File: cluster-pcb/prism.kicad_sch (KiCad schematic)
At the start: 8 parts, among them J501 Conn_01x04_P3.5mm_TBH_Horizon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, U501 Interface_RS485_MAX13431E, U502 TPS1H200AQDGNRQ1

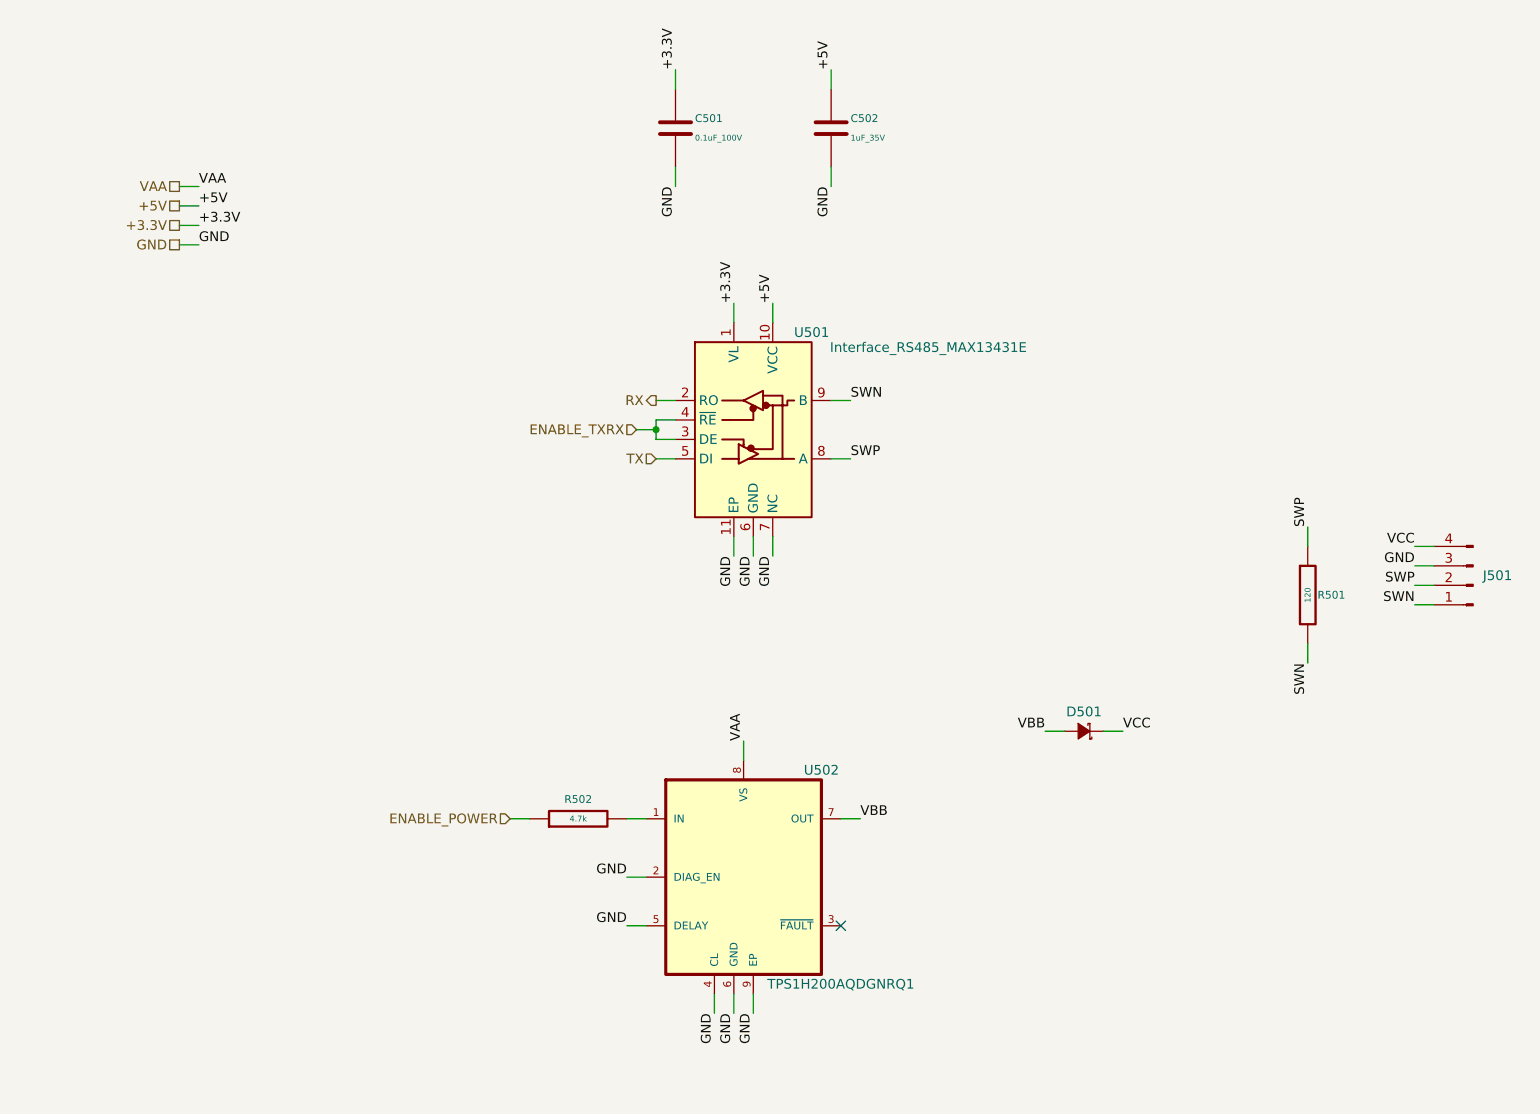
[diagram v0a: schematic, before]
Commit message: First SPI changes
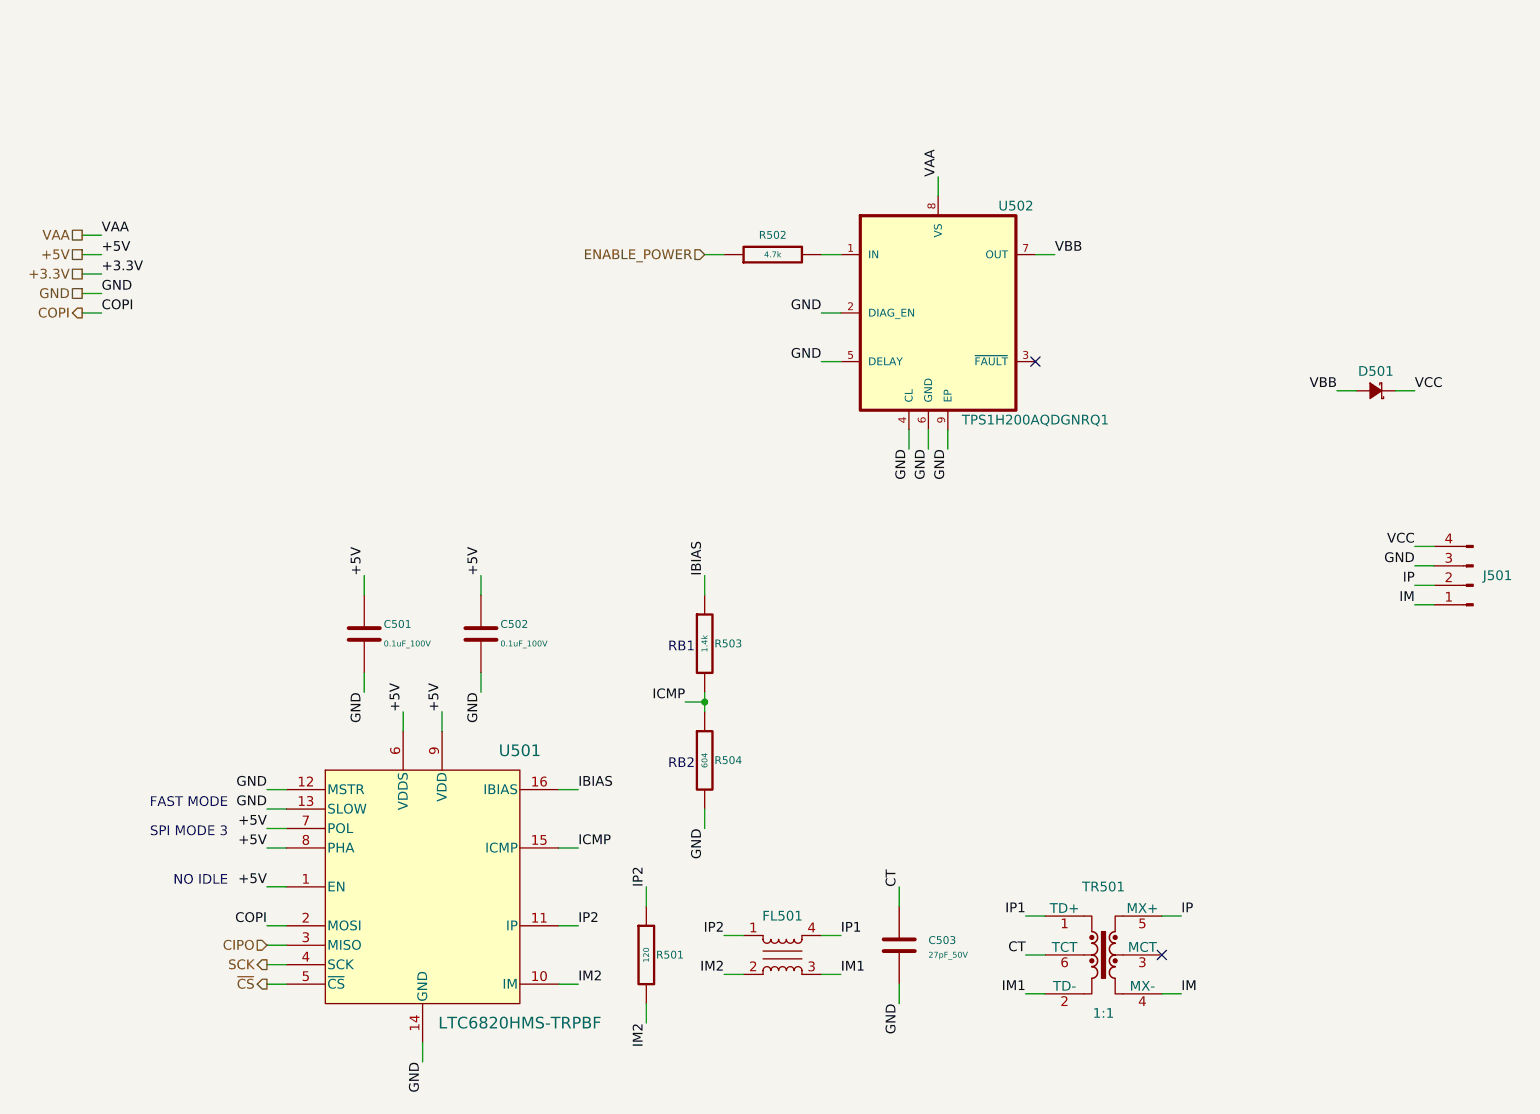
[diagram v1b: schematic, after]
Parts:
- removed C502: 1uF_35V, Janelia:C_0402_1005Metric, symbol Janelia:C_1uF_35V_0402
- removed U501: Interface_RS485_MAX13431E, Janelia:21-0137I_T1033-1_MXM, symbol Janelia:Interface_RS485_MAX13431E
- added C502: 0.1uF_100V, Janelia:C_0402_1005Metric, symbol Janelia:C_0.1uF_100V_0402
- added C503: 27pF_50V, Janelia:C_0402_1005Metric, symbol Janelia:C_27pF_50V_0402
- added FL501: Choke_CMF_ACT45B-220-2P, Janelia:SMD_0-2P-TL003_TDK-L, symbol Janelia:Choke_CMF_ACT45B-220-2P
- added R503: 1.4k, Janelia:R_0402_1005Metric, symbol Janelia:R_1.4k_0402
- added R504: 604, Janelia:R_0402_1005Metric, symbol Janelia:R_604_0402
- added TR501: 1:1, Janelia:FB020G00, symbol Janelia:Transformer_Pulse_1CT{colon}1CT_SMD
- added U501: LTC6820HMS-TRPBF, Janelia:MS_05-08-1669_ADI, symbol Janelia:LTC6820HMS-TRPBF
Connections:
- net +3.3V: no longer C501.1
- net +5V: now also C501.1, C502.1, U501.1 (EN), U501.6 (VDDS), U501.7 (POL), U501.8 (PHA), U501.9 (VDD)
- net GND: now also C502.2, C503.2, R504.2, U501.12 (MSTR), U501.13 (SLOW), U501.14 (GND)
- net SWN renamed IM
- net IM: now also TR501.4 (MX-); no longer R501.2
- net SWP renamed IP
- net IP: now also TR501.5 (MX+); no longer R501.1
- new net CIPO: U501.3 (MISO)
- new net COPI: U501.2 (MOSI)
- new net CT: C503.1, TR501.6 (TCT)
- new net IBIAS: R503.1, U501.16 (IBIAS)
- new net ICMP: R503.2, R504.1, U501.15 (ICMP)
- new net IM1: FL501.3, TR501.2 (TD-)
- new net IM2: FL501.2, R501.2, U501.10 (IM)
- new net IP1: FL501.4, TR501.1 (TD+)
- new net IP2: FL501.1, R501.1, U501.11 (IP)
- new net SCK: U501.4 (SCK)
- new net ~{CS}: U501.5 (~{CS})
- no-connect marks 1 -> 2
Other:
- note added: "FAST MODE"
- note added: "NO IDLE"
- note added: "RB1"
- note added: "RB2"
- note added: "SPI MODE 3"
- moved on the sheet: D501, R502, U502
